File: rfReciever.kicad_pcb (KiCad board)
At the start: 4 copper layers, 1 x 9.6 mm, 36 parts, among them J1 MOLEX 1054440001, SW1 RF_RESET, SW2 RF_SLEEP, U2 USBLC6-2SC6, U3 FT234XD-R, U4 TPS76333DBVT, X1 DigiXBeeRX900Micro

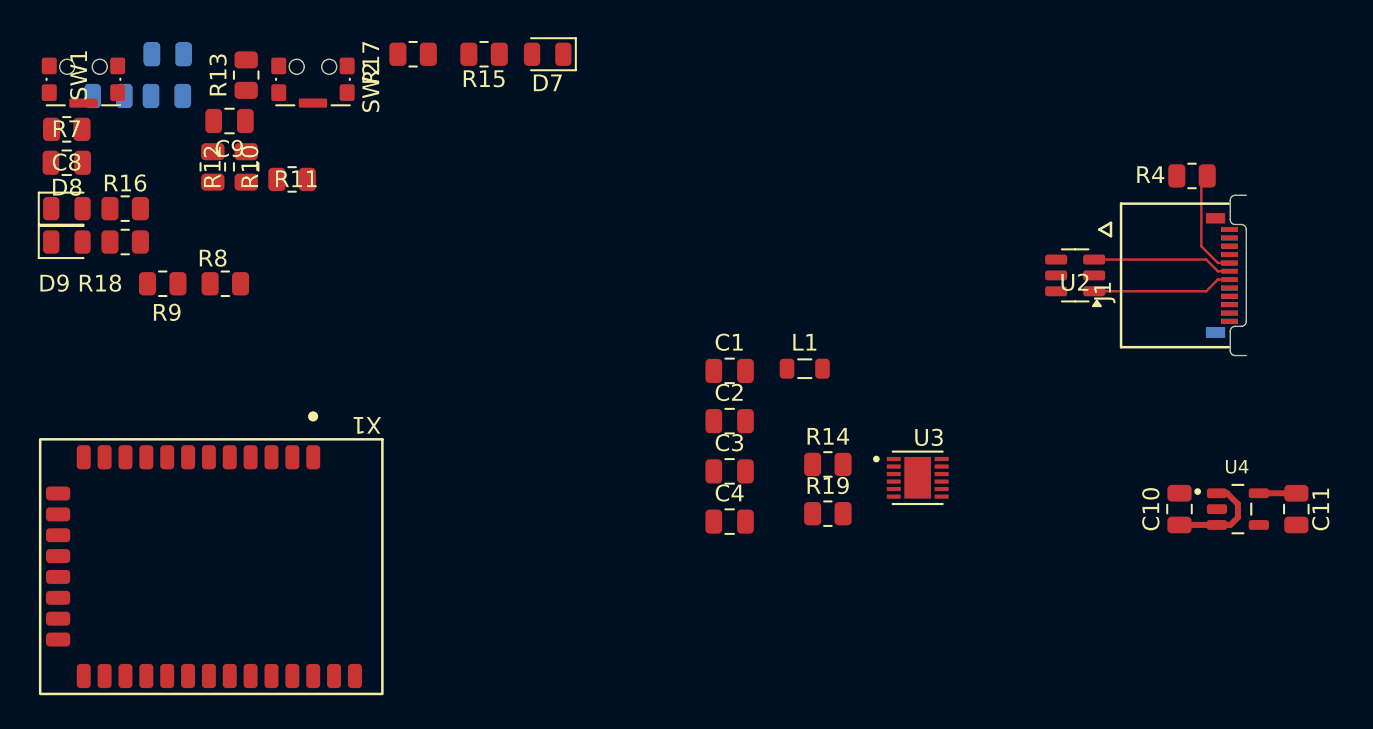
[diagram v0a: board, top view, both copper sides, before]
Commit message: gitignore + layout v3 + routing
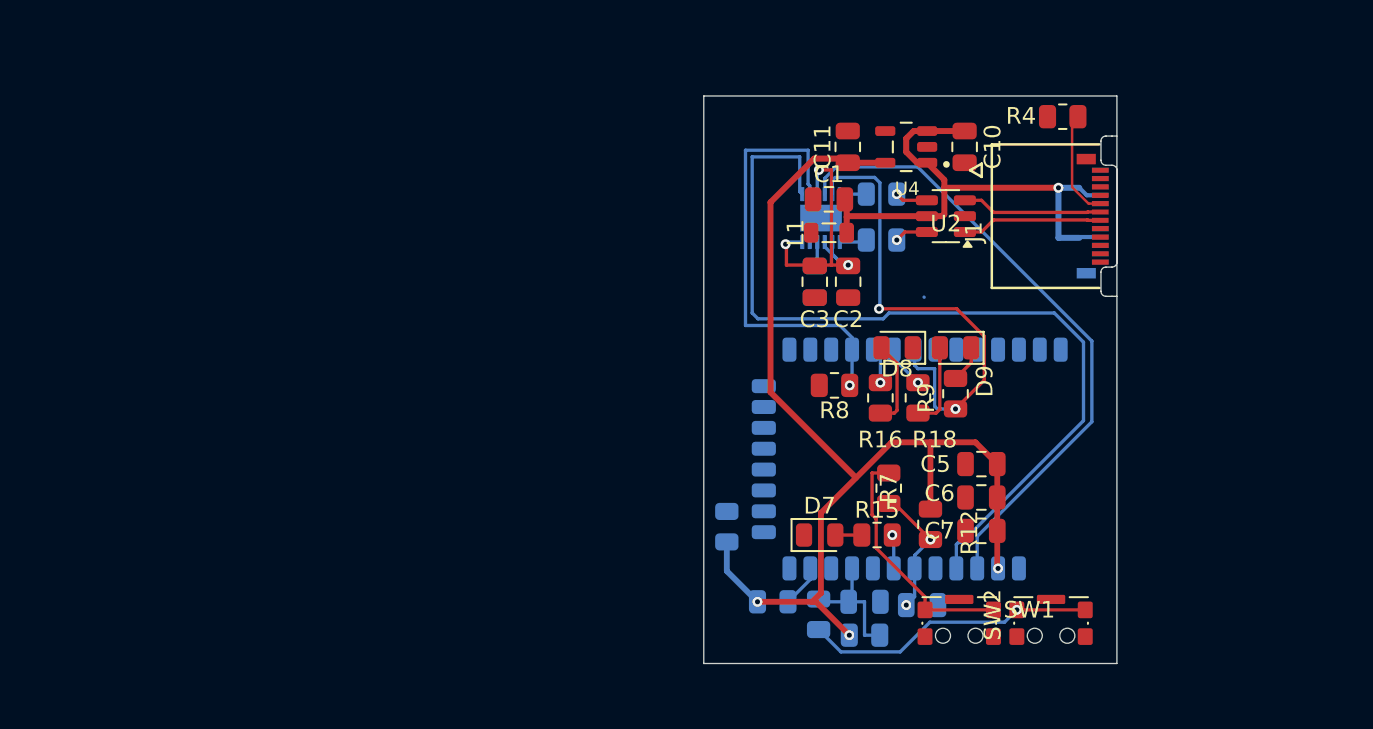
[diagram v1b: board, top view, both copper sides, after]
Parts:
- C4, C8, C9, R10, R11, R13, R14, R17, R19, U3, X1: moved to B.Cu
- C5, C6, C7: moved to F.Cu
- moved SW1 61.8 mm to (146.3, 85.8), turned to 0 degrees
- moved C8 57.7 mm to (144.1, 84.8), turned to 0 degrees
- moved C5 56.8 mm to (147.6, 76.3)
- moved C7 56.5 mm to (147.6, 80.3), turned to 180 degrees
- moved SW2 54.9 mm to (151.8, 85.8), turned to 0 degrees
- moved C6 54.4 mm to (147.6, 78.3), turned to 180 degrees
- moved R7 53.7 mm to (142.1, 77.8), turned to 90 degrees
- moved D9 53.6 mm to (146.1, 69.3), turned to 180 degrees
- moved D8 50.4 mm to (142.6, 69.3), turned to 180 degrees
- moved R18 48.4 mm to (143.8, 72.3), turned to -90 degrees
- moved R12 48.0 mm to (144.6, 79.9), turned to -90 degrees
- moved R9 47.9 mm to (146.1, 72.1), turned to 90 degrees
- moved C9 47.7 mm to (140.6, 84.6), turned to 0 degrees
- moved R13 47.1 mm to (137.9, 85.3), turned to -90 degrees
- moved R16 46.6 mm to (141.6, 72.3), turned to -90 degrees
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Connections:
- net /MLX(D+) renamed /MLXDP
- net /MLX(D-) renamed /MLXDN
- net Net-(U3-USBDM) renamed /USBDM
- net Net-(U3-USBDP) renamed /USBDP
- U3 pad 6: /VCCIO -> /FTDI_3.3V
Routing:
- net +3.3V: track 2.25 -> 66.0 mm, vias 0 -> 3
- net /RF_TXD: track 0.00 -> 52.2 mm
- net /RF_RXD: track 0.00 -> 38.0 mm
- net /UART_CTS: track 0.00 -> 29.3 mm, vias 0 -> 2
- net +5V: track 6.01 -> 32.6 mm, vias 0 -> 1
- net /UART_RTS: track 0.00 -> 26.5 mm, vias 0 -> 1
- net /RF_SW_SLEEP: track 0.00 -> 17.6 mm, vias 0 -> 1
- net /FTDI_3.3V: track 0.00 -> 17.3 mm, vias 0 -> 3
- net /RF_SW_RESET: track 0.00 -> 15.1 mm
- net /RF_RESET: track 0.00 -> 7.92 mm, vias 0 -> 2
- net /RF_SLEEP: track 0.00 -> 7.87 mm
- net /RF_D8: track 0.00 -> 5.21 mm
- net /RF_D9: track 0.00 -> 5.09 mm
- net /RF_ASSOCIATE: track 0.00 -> 2.58 mm, vias 0 -> 1
- net /RF_BOOTMODE: track 0.00 -> 2.55 mm
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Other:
- board size 1 x 9.6 mm -> 24.8 x 34 mm
